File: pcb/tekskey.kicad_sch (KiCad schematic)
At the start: 128 parts, among them J101 Conn_01x08, J102 Conn_01x08, J103 Conn_01x01_Male, J104 Conn_01x01_Male, J105 Conn_01x01_Male, J106 Conn_01x01_Male, SW101 MX_SW_HS, SW102 MX_SW_HS, SW103 MX_SW_HS, SW104 MX_SW_HS, SW105 MX_SW_HS, SW106 MX_SW_HS, SW107 MX_SW_HS, SW108 MX_SW_HS, SW109 MX_SW_HS, SW110 MX_SW_HS, SW111 MX_SW_HS, SW112 MX_SW_HS, SW113 MX_SW_HS, SW114 MX_SW_HS, SW115 MX_SW_HS, SW116 MX_SW_HS, SW117 MX_SW_HS, SW118 MX_SW_HS, SW119 MX_SW_HS, SW120 MX_SW_HS, SW121 MX_SW_HS, SW122 MX_SW_HS, SW123 MX_SW_HS, SW124 MX_SW_HS, SW125 MX_SW_HS, SW126 MX_SW_HS, SW127 MX_SW_HS, SW128 MX_SW_HS, SW129 MX_SW_HS, SW130 MX_SW_HS, SW131 MX_SW_HS, SW132 MX_SW_HS, SW133 MX_SW_HS, SW134 MX_SW_HS, SW135 MX_SW_HS, SW136 MX_SW_HS, SW1B101 MX_SW_HS, SW2B101 MX_SW_HS, SW3B101 MX_SW_HS, SW4B101 MX_SW_HS, SW51B101 MX_SW_HS, SW55B101 MX_SW_HS, SW5B101 MX_SW_HS

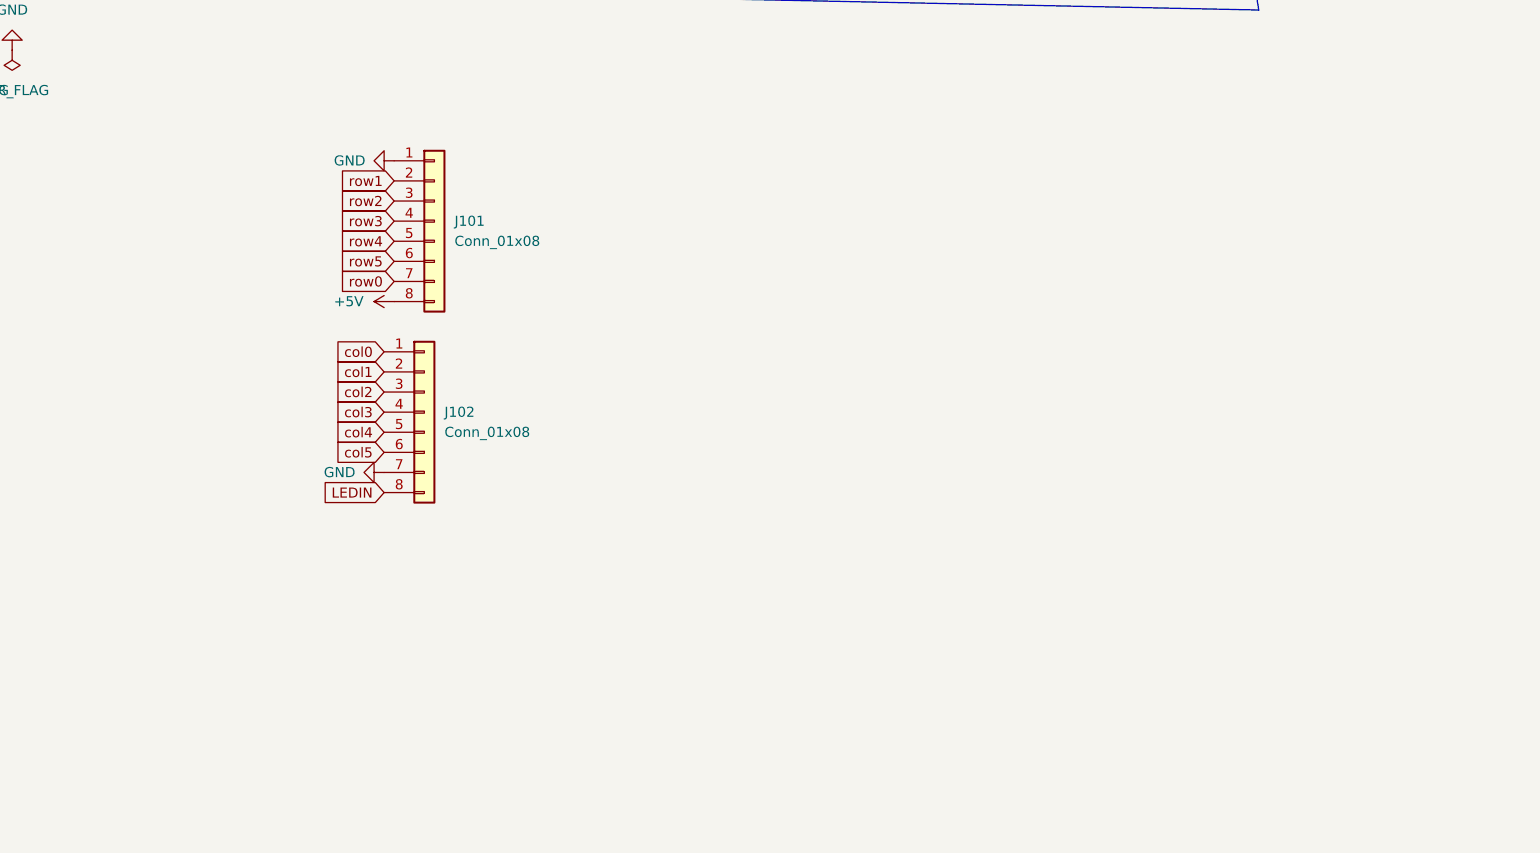
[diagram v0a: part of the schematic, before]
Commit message: adjustments
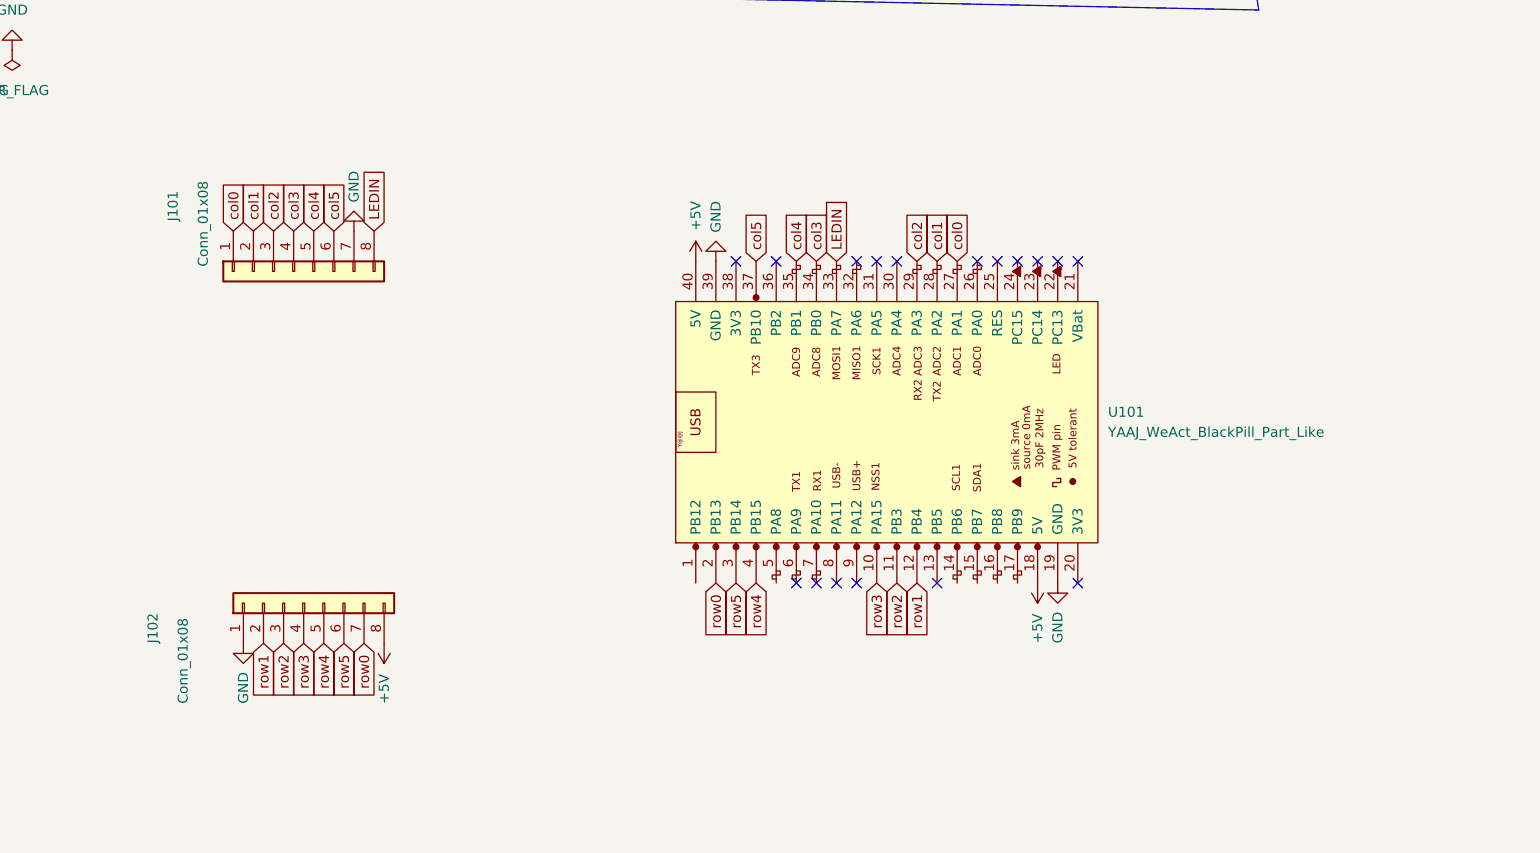
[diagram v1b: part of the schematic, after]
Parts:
- added U101: YAAJ_WeAct_BlackPill_Part_Like, Footprints:YAAJ_WeAct_BlackPill_SWD_2, symbol YAAJ_WeAct_BlackPill_Part_Like:YAAJ_WeAct_BlackPill_Part_Like
- renumbered J102 to J101, J101 to J102
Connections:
- net +5V: now also U101.18 (5V), U101.40 (5V)
- net GND: now also U101.19 (GND), U101.39 (GND)
- net LEDIN: now also U101.33 (PA7)
- net col0: now also U101.27 (PA1)
- net col1: now also U101.28 (PA2)
- net col2: now also U101.29 (PA3)
- net col3: now also U101.34 (PB0)
- net col4: now also U101.35 (PB1)
- net col5: now also U101.37 (PB10)
- net row0: now also U101.2 (PB13)
- net row1: now also U101.12 (PB4)
- net row2: now also U101.11 (PB3)
- net row3: now also U101.10 (PA15)
- net row4: now also U101.4 (PB15)
- net row5: now also U101.3 (PB14)
- no-connect marks 1 -> 18
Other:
- moved on the sheet: J101, J102
